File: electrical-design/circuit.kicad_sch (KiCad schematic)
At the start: 47 parts, among them J1 AVR-ISP-10, J2 Conn_01x03_Female, Q1 2N3906, Q2 2N3906, Q3 2N3906, Q4 2N3906, SW1 SW_Push, SW2 SW_DIP_x04, SW3 SW_Push, U1 ATmega8A-P, U2 LTC-4627JD, U3 NE555P, Y1 16MHz

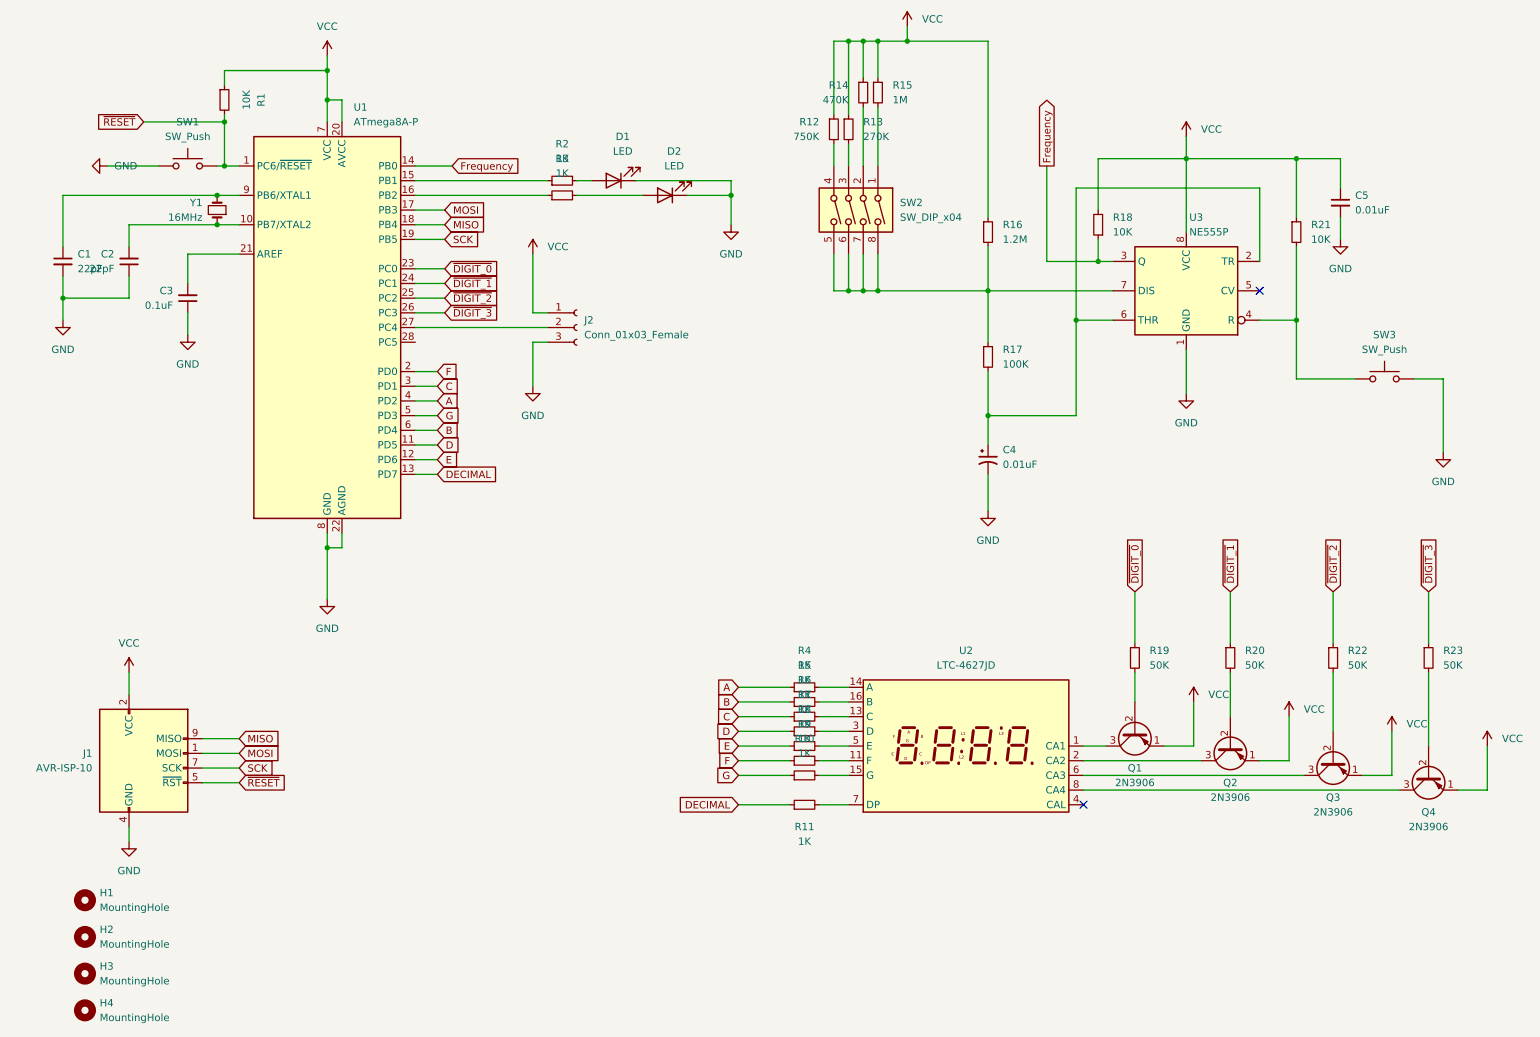
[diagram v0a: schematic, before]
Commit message: Completed Initial Design of Circuit Board
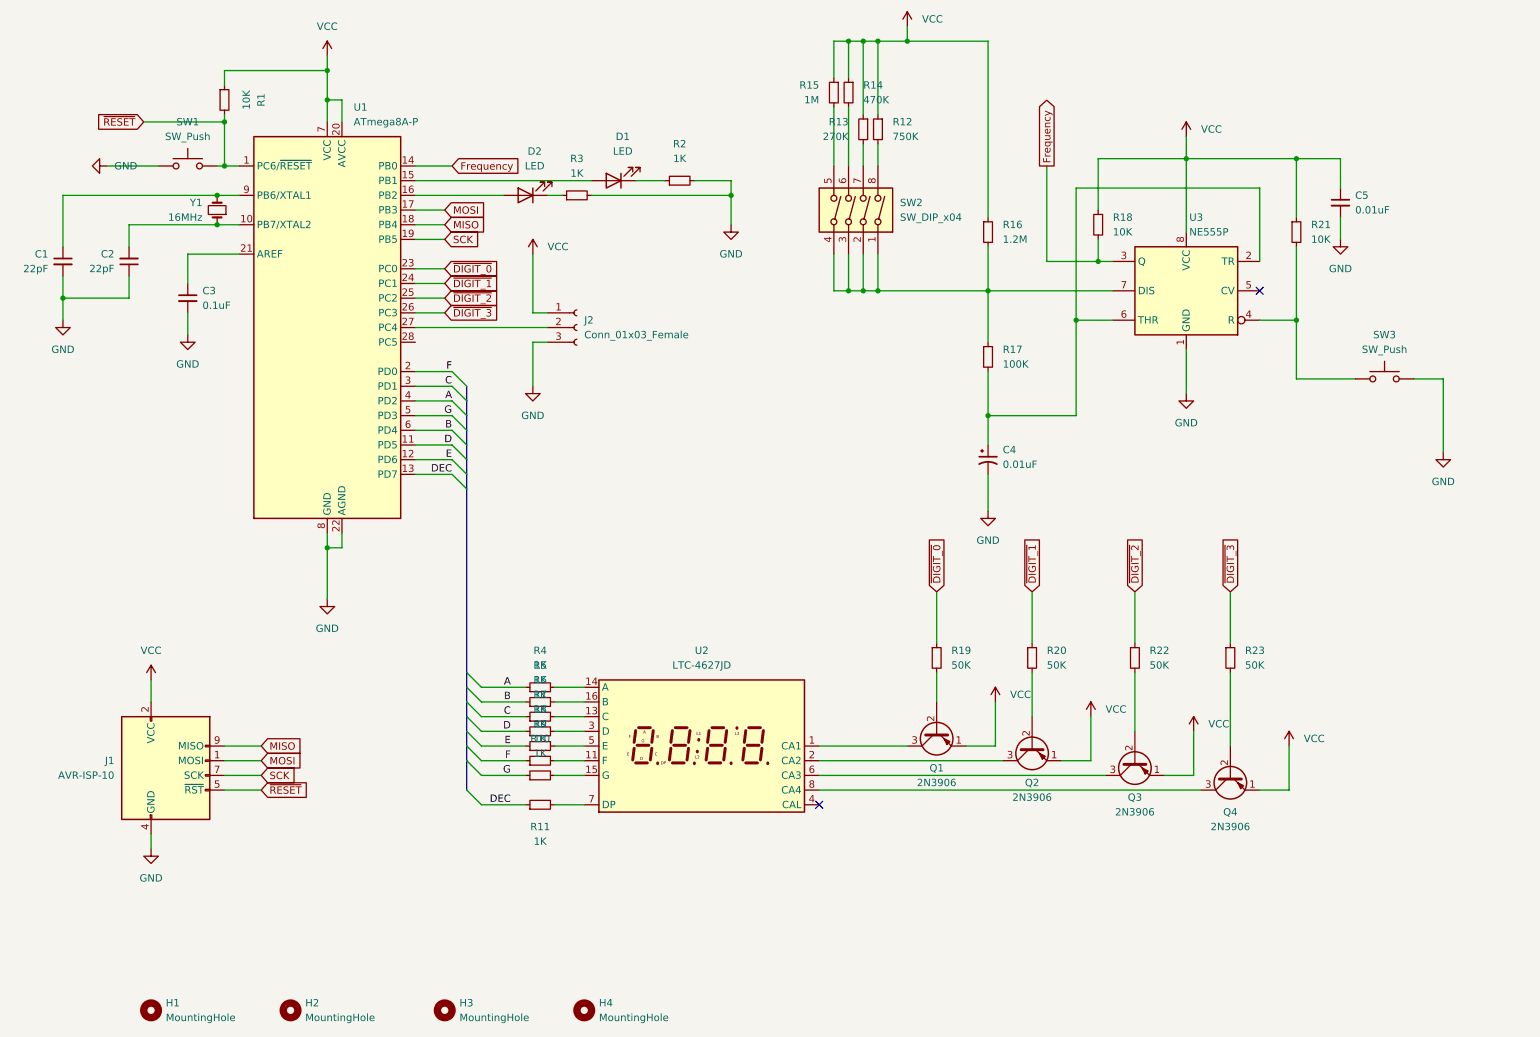
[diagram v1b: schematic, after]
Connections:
- net Frequency: now also R18.2; no longer R18.1
- net GND: now also C3.2, R2.2, R3.2; no longer C3.1, D1.1 (K), D2.1 (K)
- net VCC: now also R18.1; no longer R18.2
- net at U1.15 (PB1): now also D1.2 (A); no longer R2.1
- net at U1.16 (PB2): now also D2.2 (A); no longer R3.1
- net at U1.21 (AREF): now also C3.1; no longer C3.2
- net at SW2.1: now also R16.2, R17.1, SW2.2, SW2.3, SW2.4, U3.7 (DIS); no longer R15.2
- net at R14.2: now also SW2.6; no longer SW2.2
- net at R13.2: now also SW2.7; no longer SW2.3
- net at R12.2: now also SW2.8; no longer SW2.4
- net DECIMAL renamed DEC
- new net: R15.2, SW2.5
- new net: D2.1 (K), R3.1
- new net: D1.1 (K), R2.1
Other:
- moved on the sheet: D2, H1, H2, H3, H4, J1, Q1, Q2, Q3, Q4, R10, R11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
